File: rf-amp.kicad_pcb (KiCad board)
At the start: 2 copper layers, 38 parts, among them J1 105-1102-001, J2 105-1103-001, J3 105-1102-001, J4 Conn_Coaxial, J5 Conn_Coaxial, K1 G5V-1, Q1 MMBT3904-TP, Q2 MMBT3904-TP, Q3 MMBT3904-TP, Q4 MMBT3904-TP, Q5 MMBT3904-TP, Q6 MMBT3904-TP

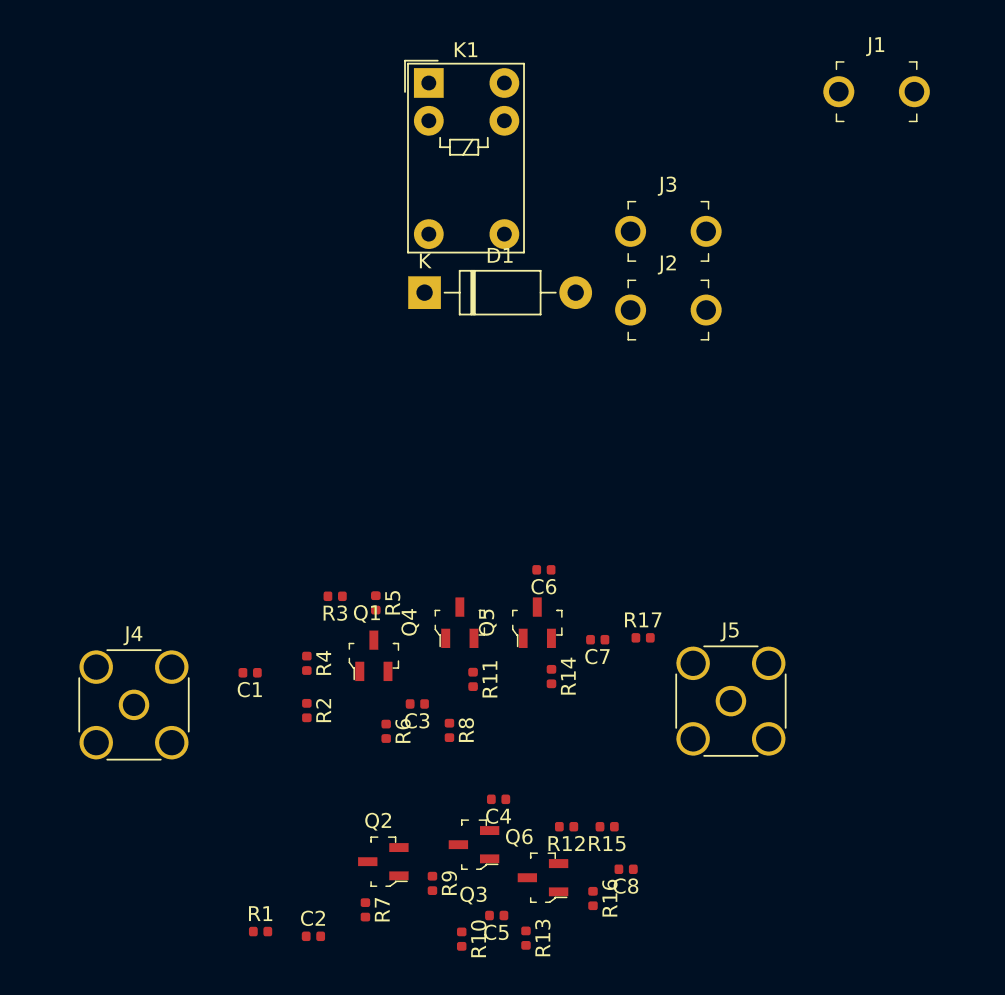
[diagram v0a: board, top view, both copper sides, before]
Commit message: Ver 1.0
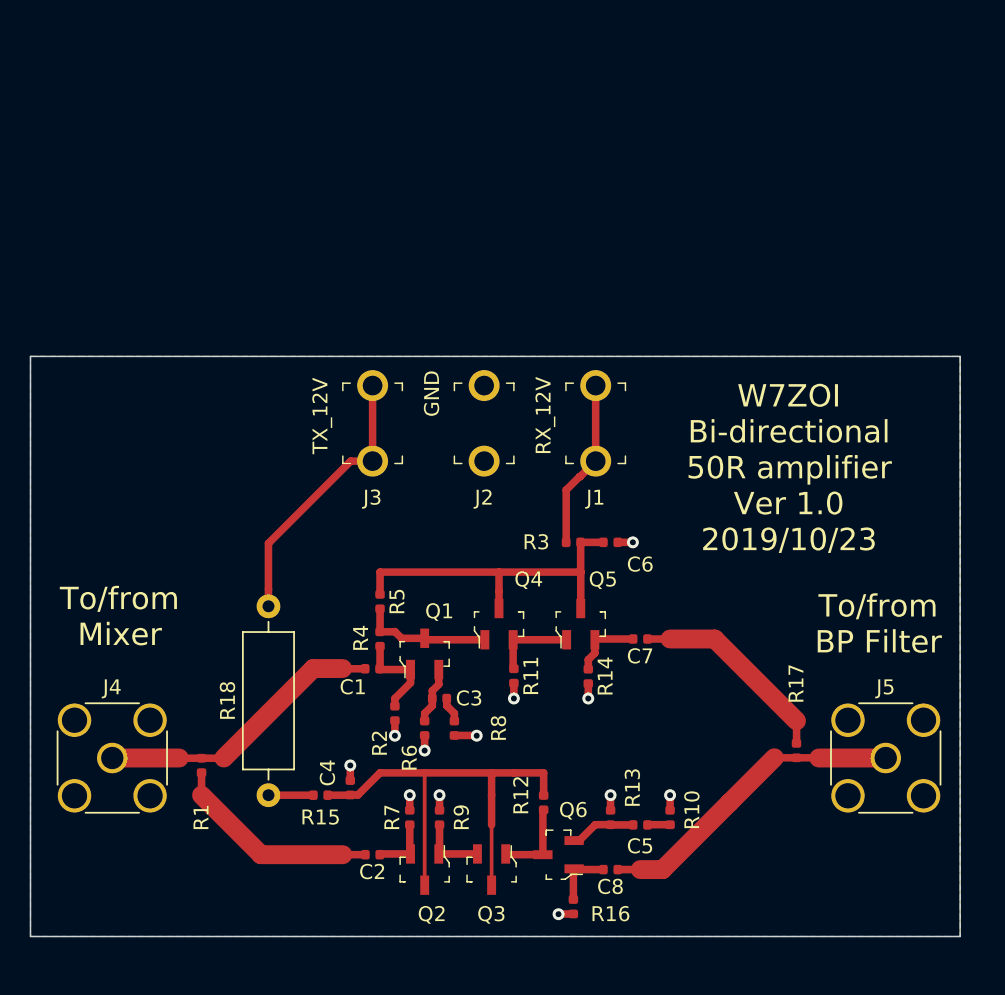
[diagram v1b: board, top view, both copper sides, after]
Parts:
- removed D1: 1N4004, Diode_THT:D_DO-41_SOD81_P10.16mm_Horizontal
- removed K1: G5V-1, Relay_THT:Relay_SPDT_Omron_G5V-1
- added R18: R_Small_US, Resistor_THT:R_Axial_DIN0309_L9.0mm_D3.2mm_P12.70mm_Horizontal, F.Cu at (125.5, 132.5)
- moved J1 29.2 mm to (147.5, 107.5), turned to 90 degrees
- moved J3 23.7 mm to (132.5, 107.5), turned to 90 degrees
- moved R15 19.4 mm to (129.0, 132.5), turned to 0 degrees
- moved R3 16.4 mm to (146.0, 115.5)
- moved R10 16.2 mm to (152.5, 134.0), turned to 90 degrees
- moved J2 14.5 mm to (140.0, 107.5), turned to 90 degrees
- moved R17 12.8 mm to (161.0, 129.5), turned to 270 degrees
- moved R1 11.9 mm to (121.0, 130.5), turned to 270 degrees
- moved C5 11.4 mm to (150.5, 134.5), turned to 0 degrees
- moved J5 11.1 mm to (167.0, 130.0)
- moved C4 10.0 mm to (131.0, 132.0), turned to 270 degrees
- moved R13 9.91 mm to (148.5, 134.0), turned to 90 degrees
- moved C1 8.22 mm to (132.5, 124.0)
- moved R7 6.89 mm to (135.0, 134.0), turned to 90 degrees
- moved C2 6.78 mm to (132.5, 136.5), turned to 180 degrees
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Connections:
- J1 pad 1: +12V -> RX_12V
- Q2 pad 2: Net-(Q2-Pad2) -> Net-(C2-Pad1)
- Q2 pad 3: Net-(C2-Pad1) -> Net-(C4-Pad2)
- Q3 pad 2: Net-(C4-Pad2) -> Net-(Q2-Pad1)
- Q3 pad 3: Net-(Q2-Pad1) -> Net-(C4-Pad2)
- Q6 pad 2: Net-(Q3-Pad1) -> Net-(C5-Pad1)
- Q6 pad 3: Net-(C5-Pad1) -> Net-(Q3-Pad1)
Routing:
- net Net-(C4-Pad2): track 0.00 -> 31.8 mm
- net Net-(C6-Pad2): track 0.00 -> 23.4 mm
- net Net-(C8-Pad1): track 0.00 -> 21.1 mm
- net Net-(C1-Pad2): track 0.00 -> 19.5 mm
- net Net-(J3-Pad1): track 0.00 -> 18.6 mm
- net Net-(C2-Pad2): track 0.00 -> 14.2 mm
- net Net-(C7-Pad1): track 0.00 -> 13.8 mm
- net GND: track 0.00 -> 12.7 mm, vias 0 -> 12
- net RX_12V: track 0.00 -> 11.4 mm
- net Net-(Q1-Pad3): track 0.00 -> 8.83 mm
- net Net-(C1-Pad1): track 0.00 -> 6.53 mm
- net Net-(Q4-Pad2): track 0.00 -> 5.57 mm
- net Net-(Q3-Pad1): track 0.00 -> 5.56 mm
- net Net-(C7-Pad2): track 0.00 -> 4.79 mm
- net Net-(Q2-Pad1): track 0.00 -> 4.59 mm
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- added copper zone on B.Cu, net GND
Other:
- board outline added: 62.5 x 39 mm
- board text added: "GND"
- board text added: "RX_12V"
- board text added: "TX_12V"
- board text added: "To/from BP Filter"
- board text added: "To/from Mixer"
- board text added: "W7ZOI Bi-directional 50R amplifier Ver 1.0 2019/10/23"
